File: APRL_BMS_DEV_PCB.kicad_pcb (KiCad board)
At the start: 4 copper layers, 129.5 x 73 mm, 73 parts, among them J1 Conn_01x04_Pin, J3 Conn_01x02_Pin, J4 Conn_01x08_Pin, J5 Conn_01x01_Pin, Q2 NPN, SW1 SW_SPDT, U1 BQ756506-Q1, U2 STM32F446RCTx, U3 ISO7741DWR, Y1 20MHz

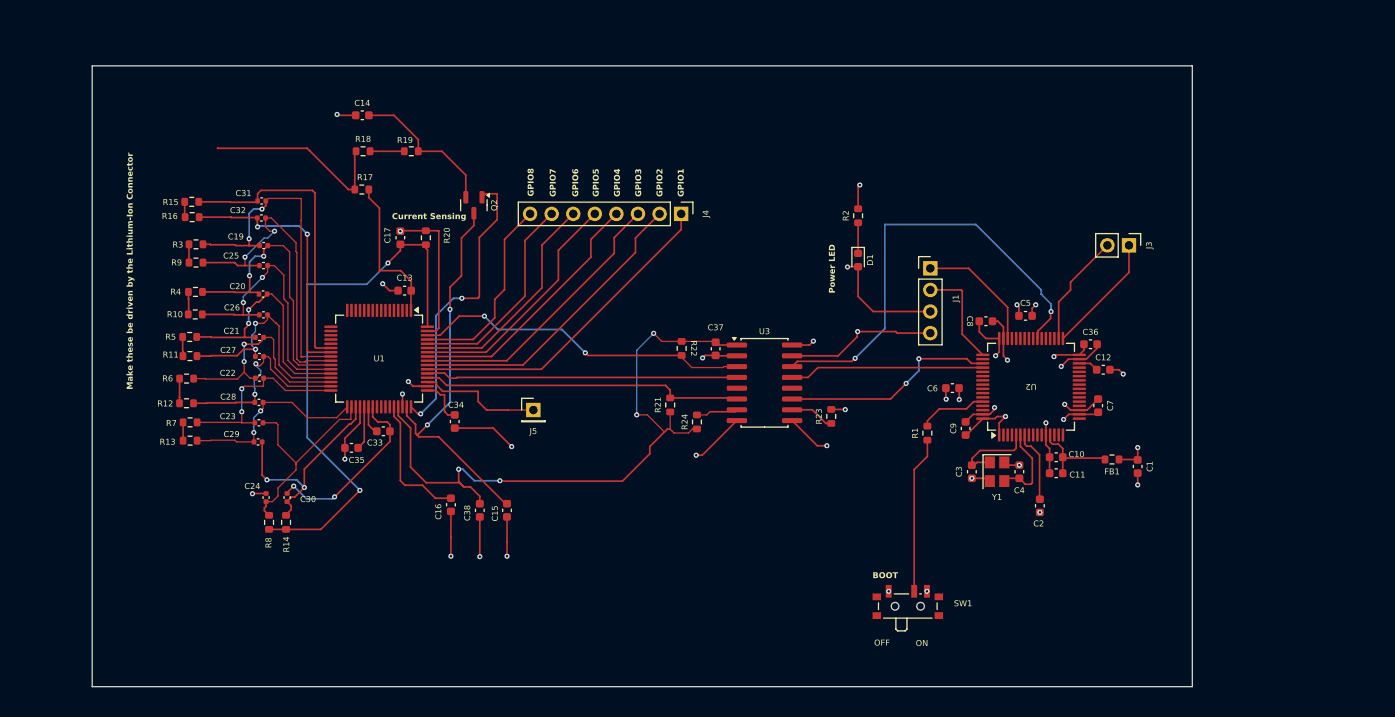
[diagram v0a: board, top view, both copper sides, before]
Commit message: Initial design COMPLETE!
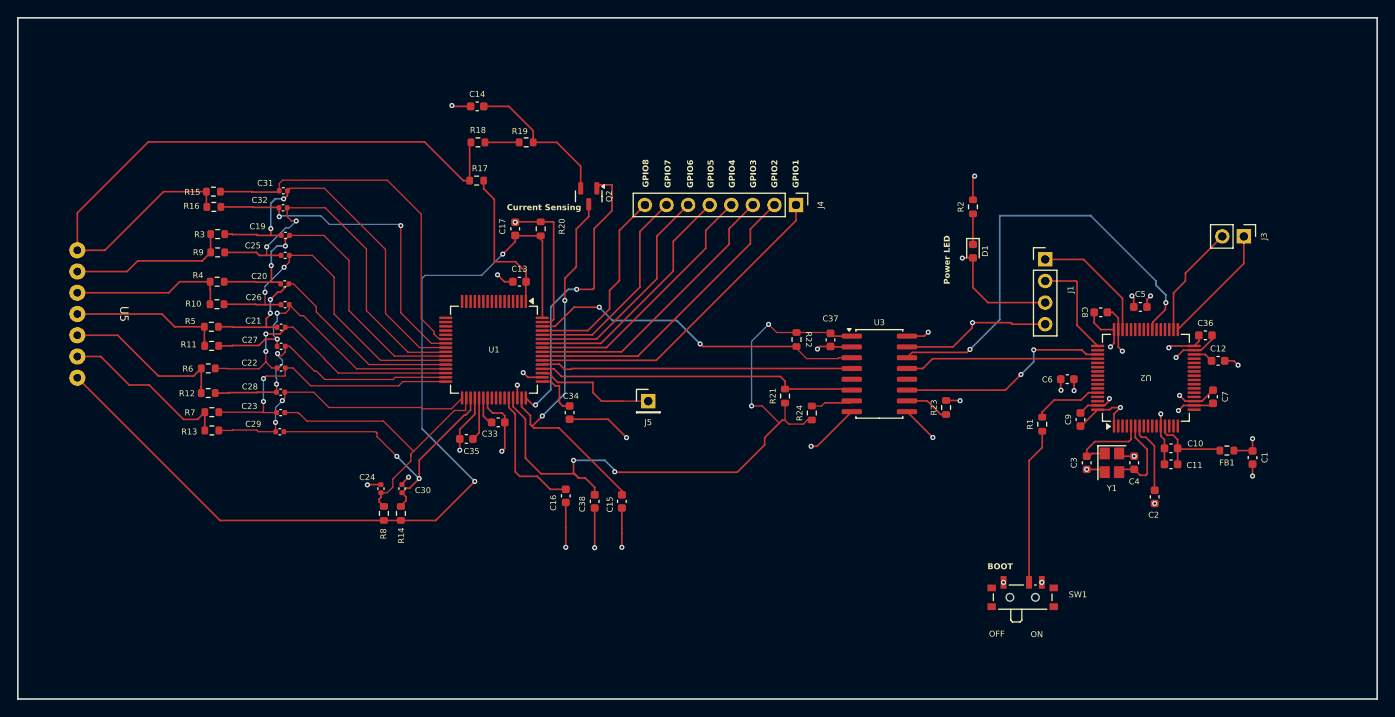
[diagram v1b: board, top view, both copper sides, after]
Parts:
- added U5: ~, Custom_Connectors:S7B-XH-A-1, F.Cu at (79.8, 84.8)
- moved C12 13.6 mm to (209.1, 90.3)
- moved C15 13.6 mm to (138.9, 106.8)
- moved C36 13.6 mm to (207.6, 87.3)
- moved C4 13.6 mm to (199.2, 102.3)
- moved C6 13.6 mm to (191.3, 92.4)
- moved D1 13.6 mm to (180.2, 77.3)
- moved FB1 13.6 mm to (210.1, 100.8)
- moved J1 13.6 mm to (188.7, 78.3)
- moved J3 13.6 mm to (212.1, 75.6)
- moved J5 13.6 mm to (142.0, 95.0)
- moved R2 13.6 mm to (180.2, 72.1)
- moved R24 13.6 mm to (161.3, 96.4)
- moved SW1 13.6 mm to (186.1, 117.8)
- moved U2 13.6 mm to (200.6, 92.3)
- moved Y1 13.6 mm to (196.6, 102.3)
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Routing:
- net /CELL_6: track 24.6 -> 80.3 mm
- net /CELL_0: track 65.5 -> 108.3 mm
- net /CELL_1: track 2.15 -> 20.6 mm
- net /CELL_2: track 2.90 -> 19.8 mm
- net /CELL_5: track 2.15 -> 18.8 mm
- net /CELL_4: track 2.63 -> 18.8 mm
- net /CELL_3: track 2.26 -> 17.8 mm
- net GND: track 152.1 -> 138.7 mm
- net /CB1: track 23.0 -> 34.4 mm
- net /VC1: track 23.2 -> 34.2 mm
- net /VC2: track 24.9 -> 35.4 mm
- net /CB0: track 25.9 -> 35.7 mm
- net /CB2: track 26.0 -> 35.2 mm
- net /VC0: track 26.5 -> 35.5 mm
- net /VC6: track 30.9 -> 39.8 mm
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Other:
- board size 129.5 x 73 mm -> 160 x 80.2 mm
- board text removed: "Make these be driven by the Lithium-Ion Connector"
